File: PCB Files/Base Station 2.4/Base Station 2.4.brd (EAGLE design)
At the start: 41.1 x 22.9 mm, 11 parts, among them U1 TXB0104, U2 CY7C65213

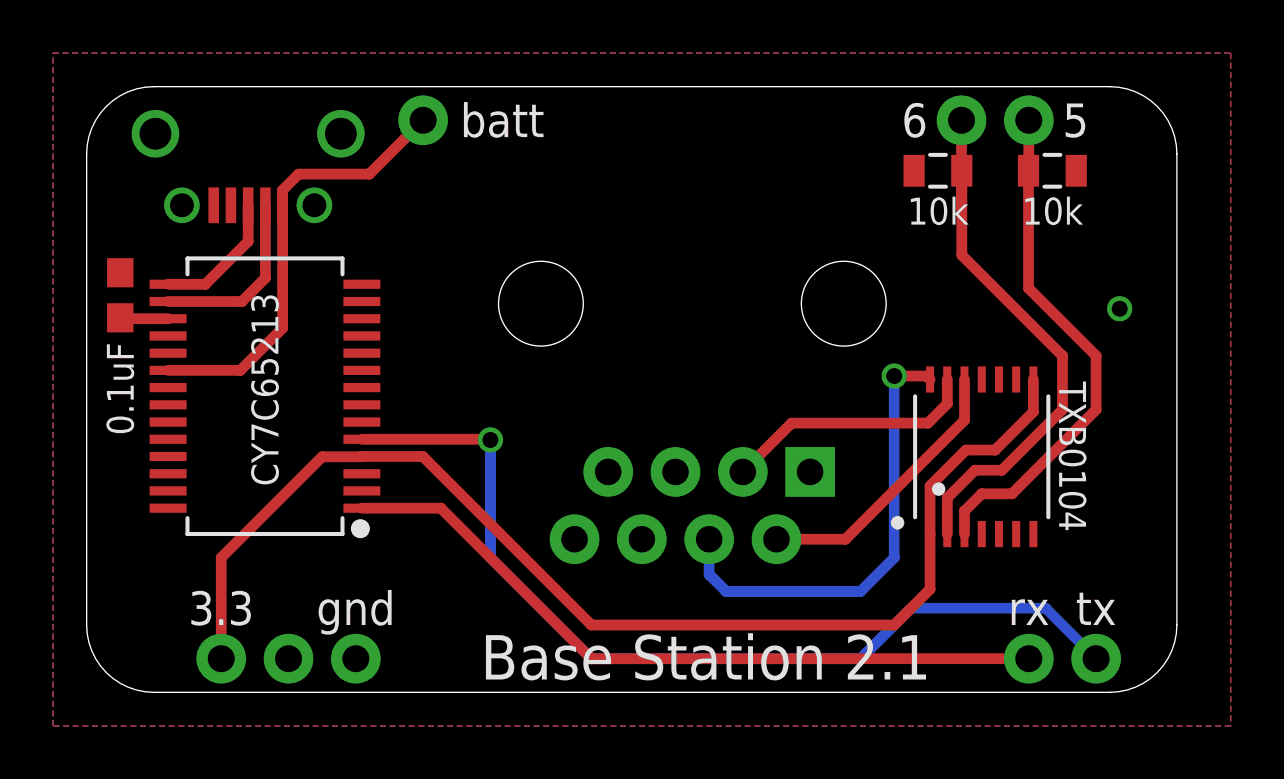
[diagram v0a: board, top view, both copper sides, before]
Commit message: Updated to latest PCB files
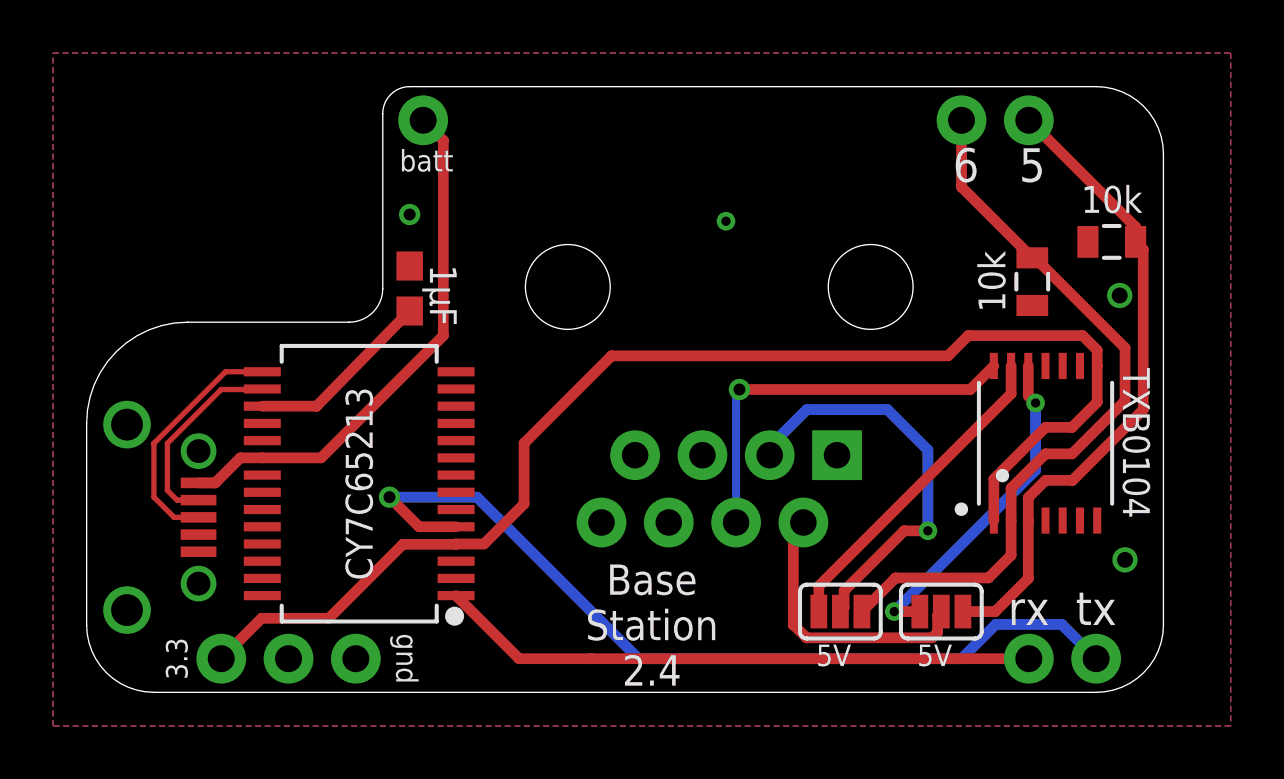
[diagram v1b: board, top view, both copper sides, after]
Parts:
- added SJ1, SJ2: (no value), SparkFun-Retired:SJ_3_PASTE2&3
- C1: value 0.1uF -> 1µF
- moved U$4 15.2 mm to (5.33, 6.60), turned to 270 degrees
- moved C1 10.9 mm to (16.0, 15.2)
- moved R4 5.49 mm to (39.5, 15.5), turned to 90 degrees
- moved U2 4.85 mm to (14.1, 7.87)
- moved R3 3.50 mm to (42.5, 17.0), turned to 0 degrees
- moved U1 2.46 mm to (40.0, 9.40)
- moved U$3 1.20 mm to (27.7, 15.3)
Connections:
- new net N$8: SJ2.3, U1.12
- new net N$9: SJ1.3, U1.13
- net N$6: now also SJ1.1
- net N$7: now also SJ2.1
- net OUT1: now also SJ1.2; no longer U1.13
- net OUT2: now also SJ2.2; no longer U1.12
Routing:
- net N$8: track 0.00 -> 12.6 mm, vias 0 -> 2
- net N$9: track 0.00 -> 12.3 mm
- net N$6: track 21.0 -> 27.9 mm
- net OUT1: track 9.76 -> 15.5 mm, vias 0 -> 1
- net N$5: track 1.82 -> 7.07 mm
- net N$7: track 19.4 -> 24.5 mm
- net N$1: track 27.5 -> 22.6 mm
- net N$3: track 5.05 -> 9.24 mm
- net BATT: track 16.6 -> 20.0 mm
- net 3.3VDC: track 45.5 -> 48.3 mm
- net 5VDC: track 17.4 -> 15.0 mm
- net N$2: track 35.3 -> 33.2 mm
- net N$4: track 6.78 -> 7.54 mm
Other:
- board size 41.1 x 22.9 mm -> 40.6 x 22.9 mm
- board text added: "5V"
- board text added: "Base Station 2.4"
- board text removed: "Base Station 2.1"
